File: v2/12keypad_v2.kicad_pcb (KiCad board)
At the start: 2 copper layers, 86.2 x 70.2 mm, 56 parts, among them J1 USB_C_Receptacle_USB2.0, SW1 SW_SPDT, SW10 KEY_MX, SW11 KEY_MX, SW2 KEY_MX, SW3 KEY_MX, SW4 KEY_MX, SW5 KEY_MX, SW6 KEY_MX, SW7 KEY_MX, SW8 KEY_MX, SW9 KEY_MX, U1 RP2040, U2 NCP1117-3.3_SOT223, U3 W25Q128JVS, Y1 12MHz

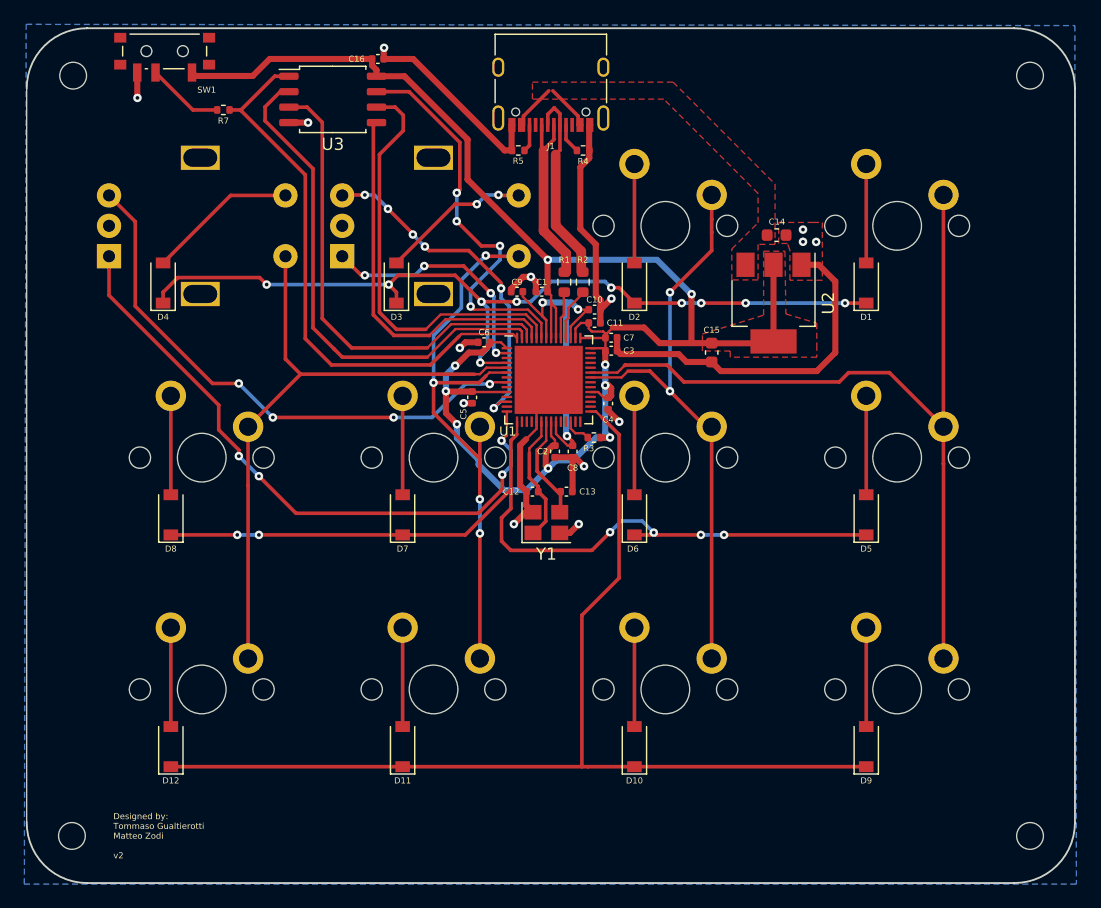
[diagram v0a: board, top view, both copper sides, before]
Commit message: general commit
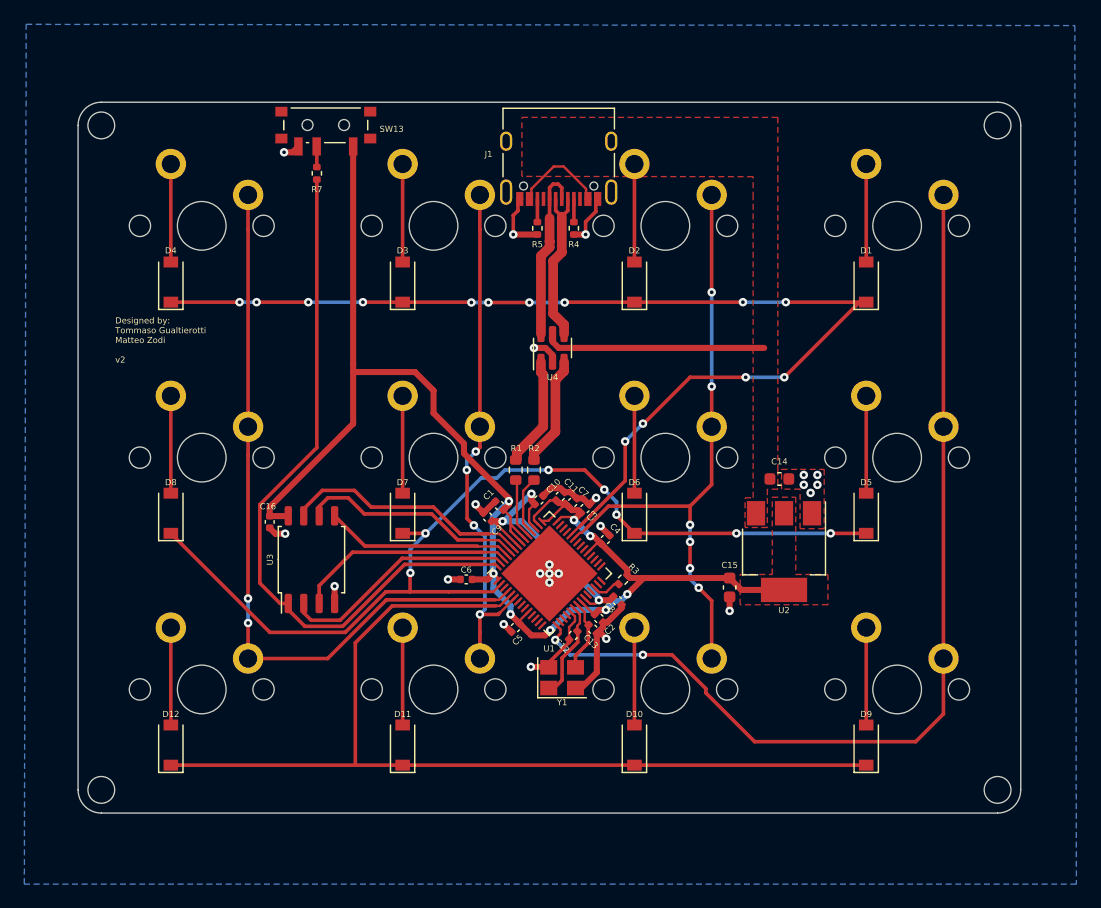
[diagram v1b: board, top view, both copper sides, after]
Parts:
- removed ENC1, ENC2: Encoder_Switch, Rotary_Encoder:RotaryEncoder_Alps_EC11E-Switch_Vertical_H20mm
- removed the SW1 at (56.4, 45.7)
- added SW13: SW_SPDT, Button_Switch_SMD:SW_SPDT_PCM12, F.Cu at (69.6, 51.7)
- added SW3: KEY_MX, Switch_Keyboard_Cherry_MX:SW_Cherry_MX_PCB_1.00u, B.Cu at (78.5, 59.7)
- added SW4: KEY_MX, Switch_Keyboard_Cherry_MX:SW_Cherry_MX_PCB_1.00u, B.Cu at (59.4, 59.7)
- added U4: USBLC6-2SC6, Package_TO_SOT_SMD:SOT-23-6, F.Cu at (88.3, 69.7)
- moved C16 39.1 mm to (65.0, 84.0), turned to -90 degrees
- moved U3 37.9 mm to (68.5, 87.1), turned to 90 degrees
- moved U2 20.4 mm to (107.3, 86.5)
- moved C14 20.0 mm to (106.9, 80.5)
- moved C6 19.5 mm to (81.2, 88.7)
- moved C15 19.4 mm to (102.8, 89.4)
- moved C5 19.3 mm to (85.2, 92.7), turned to -135 degrees
- moved C9 18.7 mm to (82.9, 83.6), turned to 135 degrees
- moved C1 17.9 mm to (83.9, 82.7), turned to 135 degrees
- moved C10 16.3 mm to (87.1, 82.2), turned to 45 degrees
- moved R2 16.0 mm to (86.7, 79.8)
- moved R1 15.9 mm to (85.2, 79.8)
- moved U1 15.9 mm to (88.0, 88.3), turned to 45 degrees
- moved C11 14.5 mm to (88.9, 81.9), turned to 45 degrees
- moved C2 14.2 mm to (92.1, 91.9), turned to -45 degrees
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- renumbered SW2 to SW1, SW9 to SW10, SW10 to SW11, SW11 to SW12, SW3 to SW2, SW4 to SW5, SW5 to SW6, SW6 to SW7, SW7 to SW8, SW8 to SW9
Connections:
- J1 pad A6: /USB_D+ -> /USB_CONN_D+
- J1 pad A7: /USB_D- -> /USB_CONN_D-
- J1 pad B6: /USB_D+ -> /USB_CONN_D+
- J1 pad B7: /USB_D- -> /USB_CONN_D-
- U1 pad 12: /ENC2_PIN_B -> unconnected-(U1-Pad12)
- U1 pad 14: /ENC1_PIN_A -> unconnected-(U1-Pad14)
- U1 pad 15: /ROW_1 -> /COL_0
- U1 pad 2: /ENC2_PIN_A -> /ROW_1
- U1 pad 29: /ROW_2 -> unconnected-(U1-Pad29)
- U1 pad 36: /COL_1 -> unconnected-(U1-Pad36)
- U1 pad 37: /COL_0 -> /COL_1
- U1 pad 38: unconnected-(U1-Pad38) -> /ROW_0
- U1 pad 4: /ROW_0 -> /COL_3
- U1 pad 5: /COL_3 -> /ROW_2
- U1 pad 8: /ENC1_PIN_B -> unconnected-(U1-Pad8)
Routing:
- net GND: track 97.9 -> 45.3 mm, vias 14 -> 24
- net /ENC1_PIN_A: track 52.4 -> 0.00 mm, vias 4 -> 0
- net /ENC1_PIN_B: track 45.5 -> 0.00 mm, vias 4 -> 0
- net /ENC2_PIN_B: track 28.1 -> 0.00 mm, vias 6 -> 0
- net /QSPI_SD1: track 42.1 -> 19.5 mm
- net +3V3: track 145.0 -> 122.5 mm, vias 9 -> 8
- net /QSPI_SD2: track 38.9 -> 18.1 mm
- net /ENC2_PIN_A: track 20.1 -> 0.00 mm, vias 4 -> 0
- net /ROW_0: track 71.5 -> 91.3 mm, vias 10 -> 14
- net VBUS: track 7.96 -> 26.5 mm
- net /QSPI_SCLK: track 34.9 -> 18.7 mm
- net /QSPI_SD0: track 31.3 -> 15.6 mm
- net /USB_CONN_D+: track 0.00 -> 14.5 mm
- net /USB_CONN_D-: track 0.00 -> 13.6 mm
- net /QSPI_SD3: track 33.1 -> 20.5 mm, vias 4 -> 0
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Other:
- board size 86.2 x 70.2 mm -> 77.5 x 58.4 mm
- board text added: "Height: 58.420 mm"
- board text added: "Width: 77.474 mm"
- board text removed: "3V3 OUT"
- board text removed: "<---- plate height 70.25 mm ---->"
- board text removed: "<---- plate width = 86.15 mm ---->"
- board text removed: "radius 3.81 mm"
